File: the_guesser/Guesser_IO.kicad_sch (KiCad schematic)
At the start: 25 parts, among them J1 Screw_Terminal_01x06, J4 Screw_Terminal_01x06, J7 USB_C_Receptacle_USB2.0_16P, Q1 AS2312, Q2 AS2312, Q3 AS2312, Q4 AS2312, Q5 AS2312, Q6 AS2312, U13 TPD4S014DSQR, U60 FUSB307BMPX

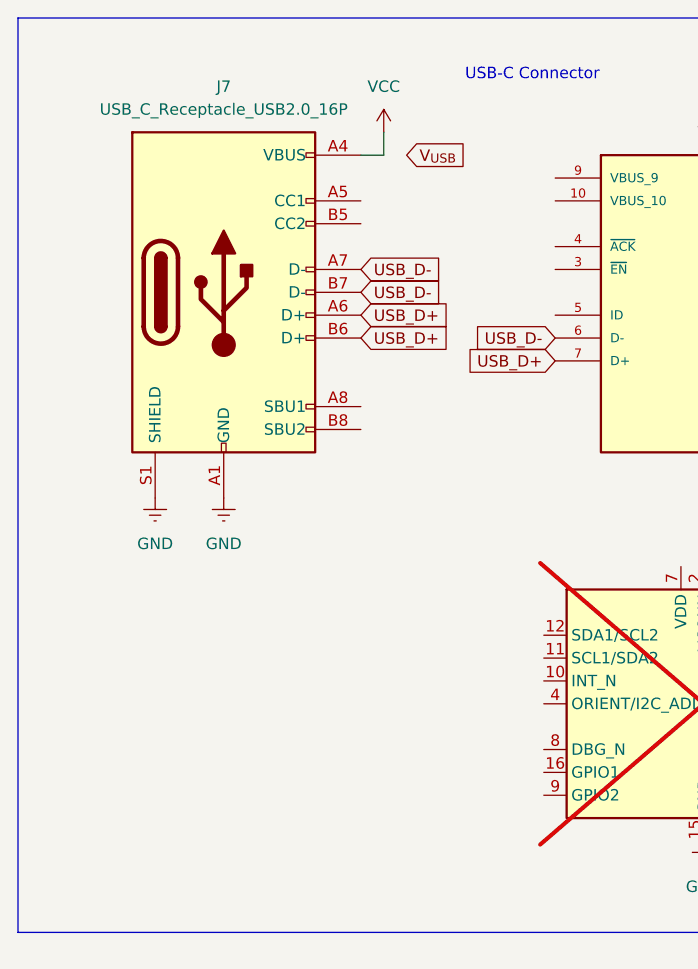
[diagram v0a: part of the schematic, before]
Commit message: Started Timer Programmer
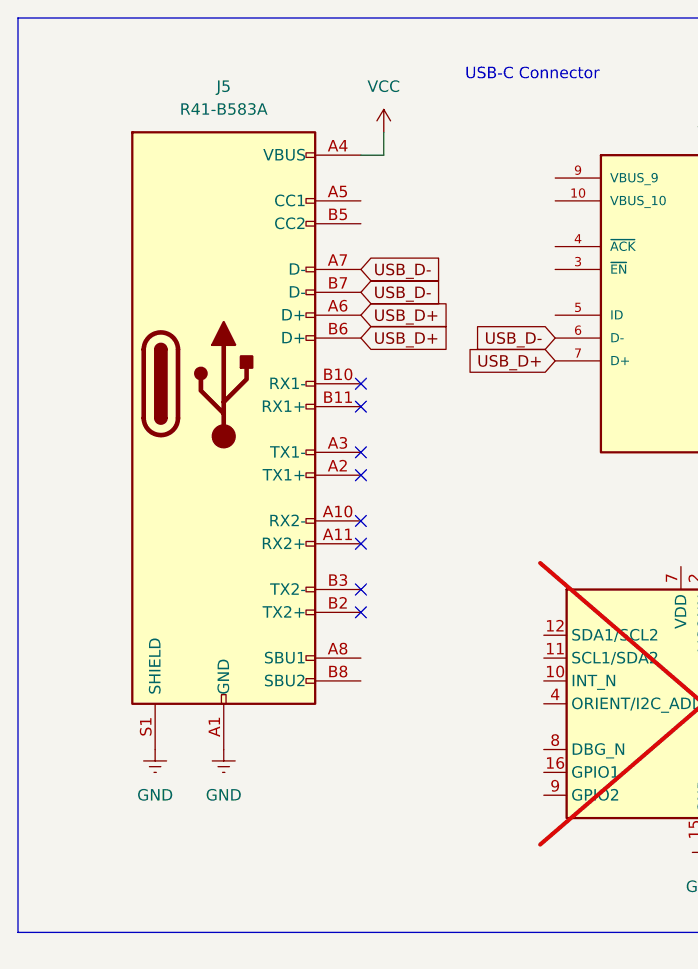
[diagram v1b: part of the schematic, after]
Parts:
- removed J7: USB_C_Receptacle_USB2.0_16P, Connector_USB:USB_C_Receptacle_GCT_USB4110, symbol Connector:USB_C_Receptacle_USB2.0_16P
- added J5: R41-B583A, locals_but_working_PLEASE:CONN_R41-B583A_MIT, symbol Connector:USB_C_Receptacle
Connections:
- net GND: now also J5.A1 (GND), J5.A12 (GND), J5.B1 (GND), J5.B12 (GND), J5.S1 (SHIELD)
- net USB_D+: now also J5.A6 (D+), J5.B6 (D+)
- net USB_D-: now also J5.A7 (D-), J5.B7 (D-)
- net VCC: now also J5.A4 (VBUS), J5.A9 (VBUS), J5.B4 (VBUS), J5.B9 (VBUS)
- no-connect marks 0 -> 8
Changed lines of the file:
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@@
 		(color 0 0 0 0)
 	)
+	(no_connect
+		(at 50.8 60.96)
+	)
+	(no_connect
+		(at 50.8 76.2)
+	)
+	(no_connect
+		(at 50.8 55.88)
+	)
+	(no_connect
+		(at 50.8 78.74)
+	)
+	(no_connect
+		(at 50.8 68.58)
+	)
+	(no_connect
+		(at 50.8 71.12)
+	)
+	(no_connect
+		(at 50.8 63.5)
+	)
+	(no_connect
+		(at 50.8 53.34)
+	)
 	(wire
 		(pts
@@
 		)
 	)
-	(global_label "V_{USB}"
-		(shape input)
-		(at 55.88 27.94 0)
-		(fields_autoplaced yes)
-		(effects
-			(font
-				(size 1.27 1.27)
-			)
-			(justify left)
-		)
-		(property "Intersheetrefs" "${INTERSHEET_REFS}"
-			(at 63.0526 27.94 0)
-			(effects
-				(font
-					(size 1.27 1.27)
-				)
-				(justify left)
-				(hide yes)
-			)
-		)
-	)
 	(global_label "C_{4}"
 		(shape input)
@@
 	(symbol
 		(lib_id "power:Earth")
-		(at 27.94 66.04 0)
+		(at 27.94 93.98 0)
 		(unit 1)
 		(exclude_from_sim no)
@@
 		(fields_autoplaced yes)
 		(property "Reference" "#PWR045"
-			(at 27.94 72.39 0)
+			(at 27.94 100.33 0)
 			(effects
 				(font
@@
 		)
 		(property "Value" "GND"
-			(at 27.94 71.12 0)
+			(at 27.94 99.06 0)
 			(effects
 				(font
@@
 		)
 		(property "Footprint" ""
-			(at 27.94 66.04 0)
+			(at 27.94 93.98 0)
 			(effects
 				(font
@@
 		)
 		(property "Datasheet" "~"
-			(at 27.94 66.04 0)
+			(at 27.94 93.98 0)
 			(effects
 				(font
@@
 		)
 		(property "Description" "Power symbol creates a global label with name \"Earth\""
-			(at 27.94 66.04 0)
+			(at 27.94 93.98 0)
 			(effects
 				(font
@@
 	)
 	(symbol
-		(lib_id "Connector:USB_C_Receptacle_USB2.0_16P")
-		(at 35.56 43.18 0)
-		(unit 1)
-		(exclude_from_sim no)
-		(in_bom yes)
-		(on_board yes)
-		(dnp no)
-		(fields_autoplaced yes)
-		(property "Reference" "J7"
-			(at 35.56 20.32 0)
-			(effects
-				(font
-					(size 1.27 1.27)
-				)
-			)
-		)
-		(property "Value" "USB_C_Receptacle_USB2.0_16P"
-			(at 35.56 22.86 0)
-			(effects
-				(font
-					(size 1.27 1.27)
-				)
-			)
-		)
-		(property "Footprint" "Connector_USB:USB_C_Receptacle_GCT_USB4110"
-			(at 39.37 43.18 0)
-			(effects
-				(font
-					(size 1.27 1.27)
-				)
-				(hide yes)
-			)
-		)
-		(property "Datasheet" "https://www.usb.org/sites/default/files/documents/usb_type-c.zip"
-			(at 39.37 43.18 0)
-			(effects
-				(font
-					(size 1.27 1.27)
-				)
-				(hide yes)
-			)
-		)
-		(property "Description" "USB 2.0-only 16P Type-C Receptacle connector"
-			(at 35.56 43.18 0)
-			(effects
-				(font
-					(size 1.27 1.27)
-				)
-				(hide yes)
-			)
-		)
-		(pin "B12"
-		)
-		(pin "A5"
-		)
-		(pin "B7"
-		)
-		(pin "A7"
-		)
-		(pin "B8"
-		)
-		(pin "A12"
-		)
-		(pin "S1"
-		)
-		(pin "B1"
-		)
-		(pin "B6"
-		)
-		(pin "B5"
-		)
-		(pin "A9"
-		)
-		(pin "A1"
-		)
-		(pin "A6"
-		)
-		(pin "A8"
-		)
-		(pin "A4"
-		)
-		(pin "B4"
-		)
-		(pin "B9"
-		)
-		(instances
-			(project "the_guesser"
-				(path "/473e3a2e-6c5e-4995-af4a-e4bf1449cab0/0bcaec57-f6d5-41f0-b678-342e153337b7"
-					(reference "J7")
-					(unit 1)
-				)
-			)
-		)
-	)
-	(symbol
 		(lib_id "Connector:Screw_Terminal_01x04")
 		(at 228.6 43.18 0)
@@
 	)
 	(symbol
+		(lib_id "Connector:USB_C_Receptacle")
+		(at 35.56 53.34 0)
+		(unit 1)
+		(exclude_from_sim no)
+		(in_bom yes)
+		(on_board yes)
+		(dnp no)
+		(fields_autoplaced yes)
+		(property "Reference" "J5"
+			(at 35.56 20.32 0)
+			(effects
+				(font
+					(size 1.27 1.27)
+				)
+			)
+		)
+		(property "Value" "R41-B583A"
+			(at 35.56 22.86 0)
+			(effects
+				(font
+					(size 1.27 1.27)
+				)
+			)
+		)
+		(property "Footprint" "locals_but_working_PLEASE:CONN_R41-B583A_MIT"
+			(at 39.37 53.34 0)
+			(effects
+				(font
+					(size 1.27 1.27)
+				)
+				(hide yes)
+			)
+		)
+		(property "Datasheet" "https://www.usb.org/sites/default/files/documents/usb_type-c.zip"
+			(at 39.37 53.34 0)
+			(effects
+				(font
+					(size 1.27 1.27)
+				)
+				(hide yes)
+			)
+		)
+		(property "Description" "USB Full-Featured Type-C Receptacle connector"
+			(at 35.56 53.34 0)
+			(effects
+				(font
+					(size 1.27 1.27)
+				)
+				(hide yes)
+			)
+		)
+		(property "DKPN" "2508-R41-B583ACT-ND"
+			(at 35.56 53.34 0)
+			(effects
+				(font
+					(size 1.27 1.27)
+				)
+				(hide yes)
+			)
+		)
+		(pin "A5"
+		)
+		(pin "B8"
+		)
+		(pin "A6"
+		)
+		(pin "A4"
+		)
+		(pin "S1"
+		)
+		(pin "B10"
+		)
+		(pin "A1"
+		)
+		(pin "A7"
+		)
+		(pin "B6"
+		)
+		(pin "A3"
+		)
+		(pin "A9"
+		)
+		(pin "B3"
+		)
+		(pin "A2"
+		)
+		(pin "B9"
+		)
+		(pin "A12"
+		)
+		(pin "B11"
+		)
+		(pin "B12"
+		)
+		(pin "A8"
+		)
+		(pin "B1"
+		)
+		(pin "A11"
+		)
+		(pin "B2"
+		)
+		(pin "B7"
+		)
+		(pin "B4"
+		)
+		(pin "A10"
+		)
+		(pin "B5"
+		)
+		(instances
+			(project "the_guesser"
+				(path "/473e3a2e-6c5e-4995-af4a-e4bf1449cab0/0bcaec57-f6d5-41f0-b678-342e153337b7"
+					(reference "J5")
+					(unit 1)
+				)
+			)
+		)
+	)
+	(symbol
 		(lib_id "Device:LED")
 		(at 219.71 114.3 180)
@@
 	(symbol
 		(lib_id "power:Earth")
-		(at 35.56 66.04 0)
+		(at 35.56 93.98 0)
 		(unit 1)
 		(exclude_from_sim no)
@@
 		(fields_autoplaced yes)
 		(property "Reference" "#PWR046"
-			(at 35.56 72.39 0)
+			(at 35.56 100.33 0)
 			(effects
 				(font
@@
 		)
 		(property "Value" "GND"
-			(at 35.56 71.12 0)
+			(at 35.56 99.06 0)
 			(effects
 				(font
@@
 		)
 		(property "Footprint" ""
-			(at 35.56 66.04 0)
+			(at 35.56 93.98 0)
 			(effects
 				(font
@@
 		)
 		(property "Datasheet" "~"
-			(at 35.56 66.04 0)
+			(at 35.56 93.98 0)
 			(effects
 				(font
@@
 		)
 		(property "Description" "Power symbol creates a global label with name \"Earth\""
-			(at 35.56 66.04 0)
+			(at 35.56 93.98 0)
 			(effects
 				(font
